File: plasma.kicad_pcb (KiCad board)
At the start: 2 copper layers, 27 parts, among them J1 Conn_01x08_Female, M1 1364_HV, Q1 MPSA42, Q2 MPSA42, Q3 MPSA42, Q4 MPSA42, Q5 MPSA42, Q6 MPSA42, U1 WeMos_D1_mini

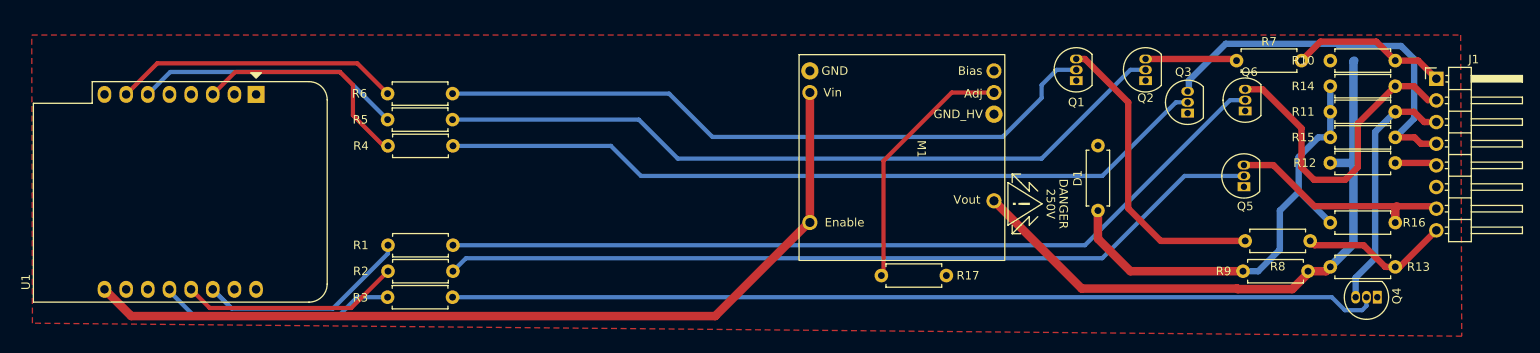
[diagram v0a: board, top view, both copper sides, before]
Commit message: playing the routing game
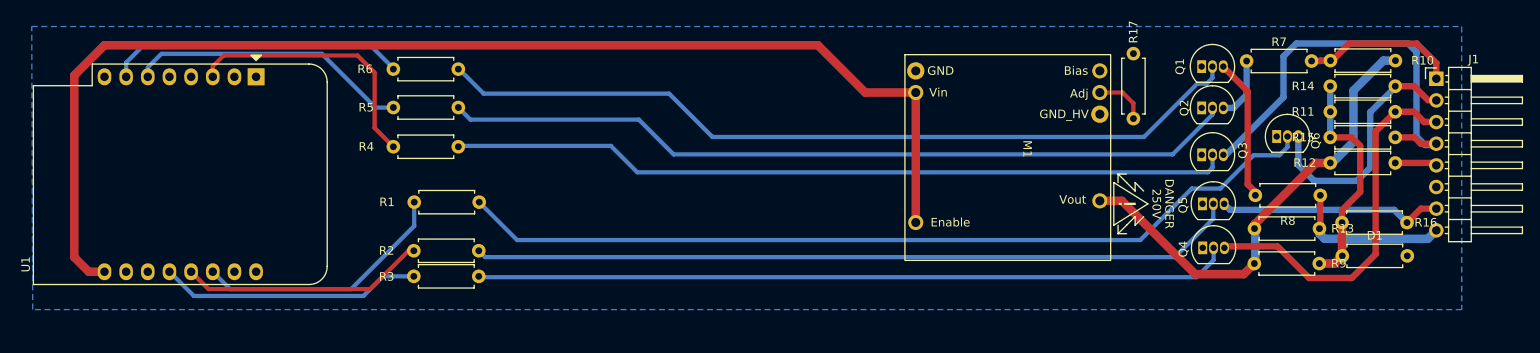
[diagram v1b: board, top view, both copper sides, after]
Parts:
- moved R17 34.8 mm to (189.1, 61.8), turned to 90 degrees
- moved D1 29.2 mm to (213.6, 77.9), turned to 0 degrees
- moved Q4 21.3 mm to (197.2, 77.0), turned to 0 degrees
- moved Q1 14.8 mm to (197.1, 55.7), turned to 0 degrees
- moved M1 12.4 mm to (162.3, 54.3)
- moved R13 9.96 mm to (203.3, 74.7)
- moved R9 8.99 mm to (210.9, 78.8), turned to 180 degrees
- moved R10 7.64 mm to (219.8, 55.0), turned to 180 degrees
- moved Q2 7.32 mm to (197.1, 60.5), turned to 0 degrees
- moved R1 5.92 mm to (104.8, 71.6)
- moved R8 5.48 mm to (203.4, 70.8)
- moved Q5 5.26 mm to (197.2, 71.8), turned to 0 degrees
- moved Q3 5.16 mm to (197.1, 66.0), turned to 0 degrees
- moved Q6 4.75 mm to (205.9, 63.9), turned to 0 degrees
- moved R3 3.93 mm to (104.7, 80.3)
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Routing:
- net +5V: track 103.8 -> 143.3 mm
- net Net-(D1-Pad1): track 54.9 -> 26.8 mm
- net Net-(M1-Pad2): track 30.0 -> 6.26 mm
- net Net-(Q4-Pad2): track 109.0 -> 88.5 mm
- net Net-(Q1-Pad3): track 35.9 -> 16.7 mm
- net VSS: track 73.1 -> 54.9 mm
- net Net-(Q1-Pad2): track 79.4 -> 95.9 mm
- net /Phase3_Cathode: track 29.4 -> 43.8 mm
- net /Phase1_Cathode: track 37.9 -> 29.6 mm
- net Net-(Q5-Pad2): track 97.4 -> 90.1 mm
- net Net-(Q2-Pad2): track 87.5 -> 93.4 mm
- net /RESET: track 27.3 -> 31.2 mm
- net /Reset_Cathode: track 45.5 -> 49.1 mm
- net Net-(Q2-Pad3): track 10.7 -> 7.34 mm
- net /P2: track 25.8 -> 28.8 mm
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- added copper zone on B.Cu, net GND
- removed copper zone on F.Cu, net GND
